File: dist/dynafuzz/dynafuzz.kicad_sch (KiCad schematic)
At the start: 54 parts, among them J1 AudioJack_IN, J2 AudioJack_OUT, J3 Jack-DC, Q1 Q_NPN, Q2 Q_NPN, Q3 Q_NPN, Q4 Q_NPN, SW1 SW_3PDT_x3

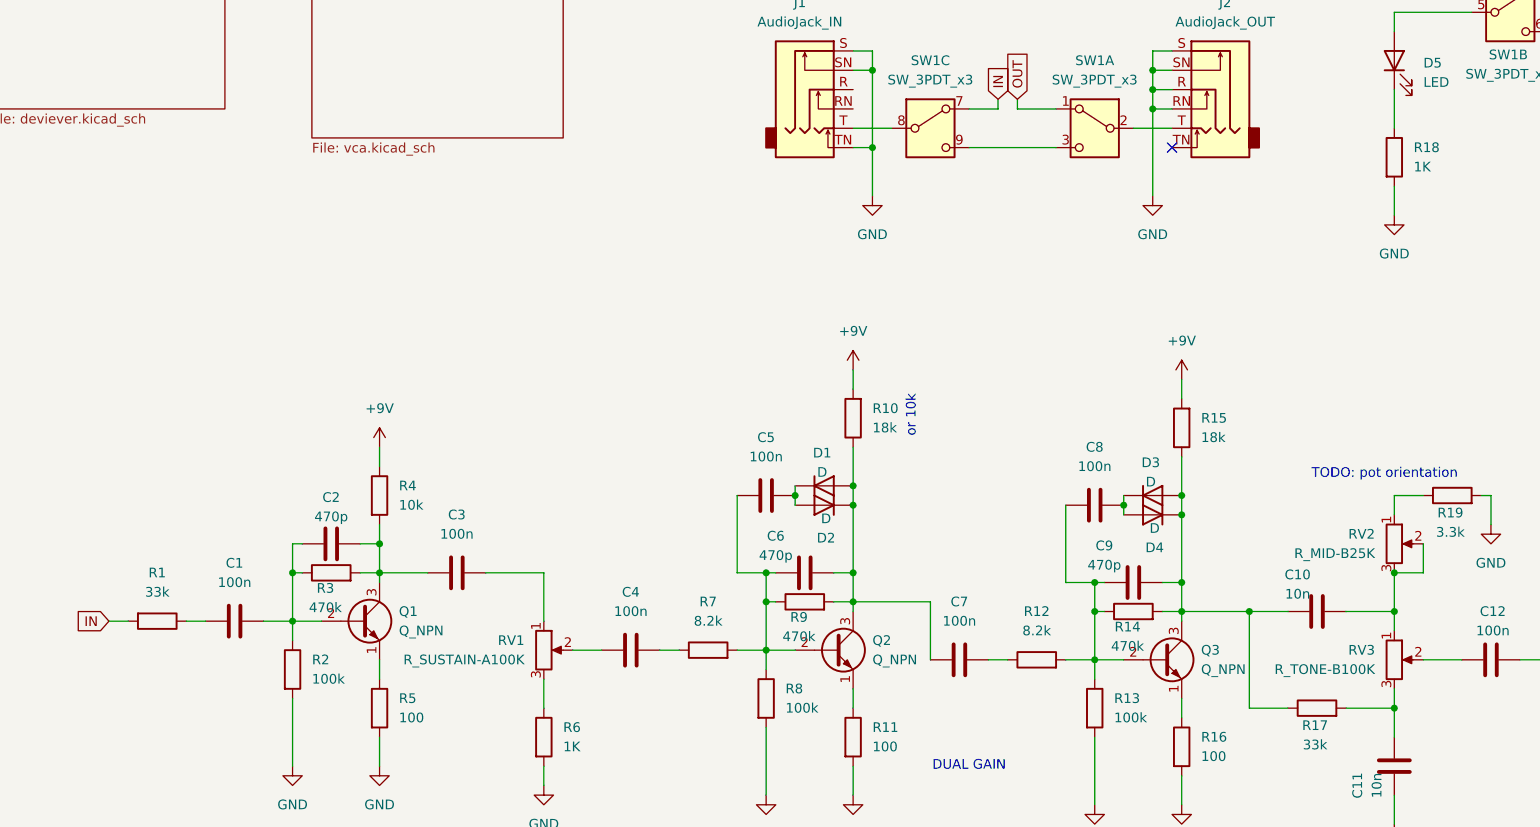
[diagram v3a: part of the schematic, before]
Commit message: update positions
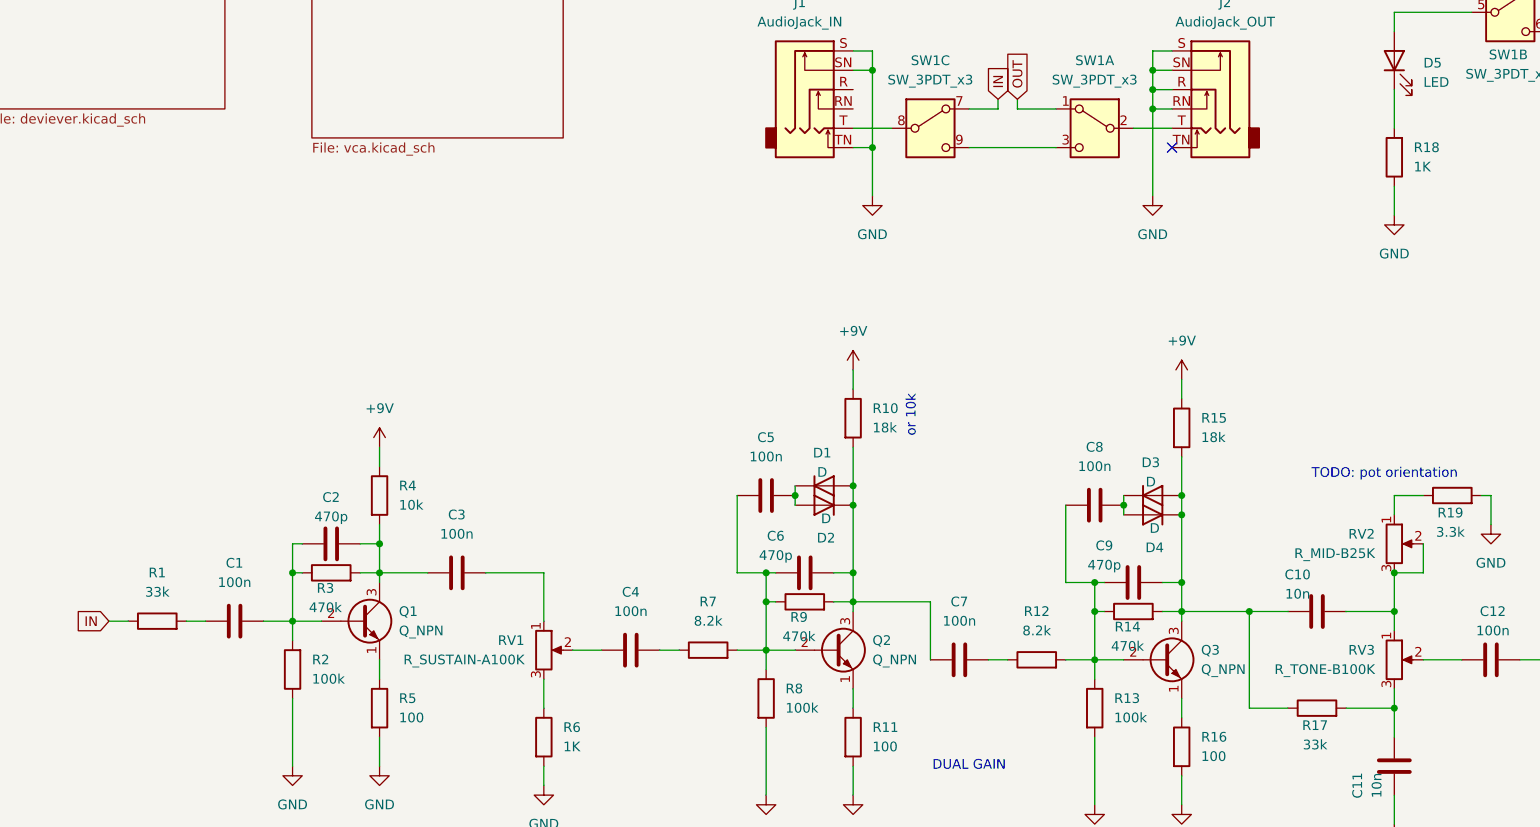
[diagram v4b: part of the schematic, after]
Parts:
- RV1, RV2, RV3, RV4: footprint Potentiometer_THT:Potentiometer_Alpha_RD901F-40-00D_Single_Vertical -> _effects_shared_footprints:Potentiometer_Alpha_RD901F-40-00D_Single_Vertical
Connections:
- net +9V: now also R10.1, R15.1; no longer R10.2, R15.2
- net GND: now also R18.1, R2.1; no longer R18.2, R2.2
- net IN: now also R1.1; no longer R1.2
- net at C10.2, C9.2, D3.2 (A)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: now also R15.2; no longer R15.1
- net at C1.2, C2.1, Q1.2 (B)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: now also R2.2; no longer R2.1
- net at C1.1: now also R1.2; no longer R1.1
- net at D5.1 (K): now also R18.2; no longer R18.1
- net at C6.2, C7.1, D1.2 (A)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: now also R10.2; no longer R10.1
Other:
- moved on the sheet: R1, R10, R15, R18, R2
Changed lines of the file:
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@@
 			)
 		)
-		(property "Footprint" "Potentiometer_THT:Potentiometer_Alpha_RD901F-40-00D_Single_Vertical"
+		(property "Footprint" "_effects_shared_footprints:Potentiometer_Alpha_RD901F-40-00D_Single_Vertical"
 			(at 88.9 109.22 0)
 			(effects
@@
 			)
 		)
-		(property "Footprint" "Potentiometer_THT:Potentiometer_Alpha_RD901F-40-00D_Single_Vertical"
+		(property "Footprint" "_effects_shared_footprints:Potentiometer_Alpha_RD901F-40-00D_Single_Vertical"
 			(at 256.54 114.3 0)
 			(effects
@@
 	(symbol
 		(lib_id "Device:R")
-		(at 55.88 111.76 0)
+		(at 55.88 111.76 180)
 		(unit 1)
 		(exclude_from_sim no)
@@
 					(size 1.27 1.27)
 				)
-				(justify left)
+				(justify right)
 			)
 		)
@@
 					(size 1.27 1.27)
 				)
-				(justify left)
+				(justify right)
 			)
 		)
 		(property "Footprint" "_project:R"
-			(at 54.102 111.76 90)
+			(at 57.658 111.76 90)
 			(effects
 				(font
@@
 			)
 		)
-		(property "Footprint" "Potentiometer_THT:Potentiometer_Alpha_RD901F-40-00D_Single_Vertical"
+		(property "Footprint" "_effects_shared_footprints:Potentiometer_Alpha_RD901F-40-00D_Single_Vertical"
 			(at 200.66 110.49 0)
 			(effects
@@
 	(symbol
 		(lib_id "Device:R")
-		(at 38.1 105.41 270)
+		(at 38.1 105.41 90)
 		(unit 1)
 		(exclude_from_sim no)
@@
 		)
 		(property "Footprint" "_project:R"
-			(at 38.1 103.632 90)
+			(at 38.1 107.188 90)
 			(effects
 				(font
@@
 			)
 		)
-		(property "Footprint" "Potentiometer_THT:Potentiometer_Alpha_RD901F-40-00D_Single_Vertical"
+		(property "Footprint" "_effects_shared_footprints:Potentiometer_Alpha_RD901F-40-00D_Single_Vertical"
 			(at 200.66 95.25 0)
 			(effects
@@
 	(symbol
 		(lib_id "Device:R")
-		(at 200.66 44.45 0)
+		(at 200.66 44.45 180)
 		(unit 1)
 		(exclude_from_sim no)
@@
 					(size 1.27 1.27)
 				)
-				(justify left)
+				(justify right)
 			)
 		)
@@
 					(size 1.27 1.27)
 				)
-				(justify left)
+				(justify right)
 			)
 		)
 		(property "Footprint" "_project:R"
-			(at 198.882 44.45 90)
+			(at 202.438 44.45 90)
 			(effects
 				(font
@@
 	(symbol
 		(lib_id "Device:R")
-		(at 129.54 78.74 180)
+		(at 129.54 78.74 0)
 		(unit 1)
 		(exclude_from_sim no)
@@
 					(size 1.27 1.27)
 				)
-				(justify right)
+				(justify left)
 			)
 		)
@@
 					(size 1.27 1.27)
 				)
-				(justify right)
+				(justify left)
 			)
 		)
 		(property "Footprint" "_project:R"
-			(at 131.318 78.74 90)
+			(at 127.762 78.74 90)
 			(effects
 				(font
@@
 	(symbol
 		(lib_id "Device:R")
-		(at 172.72 80.01 180)
+		(at 172.72 80.01 0)
 		(unit 1)
 		(exclude_from_sim no)
@@
 					(size 1.27 1.27)
 				)
-				(justify right)
+				(justify left)
 			)
 		)
@@
 					(size 1.27 1.27)
 				)
-				(justify right)
+				(justify left)
 			)
 		)
 		(property "Footprint" "_project:R"
-			(at 174.498 80.01 90)
+			(at 170.942 80.01 90)
 			(effects
 				(font
